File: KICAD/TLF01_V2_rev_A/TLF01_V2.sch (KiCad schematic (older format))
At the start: 52 parts, among them J1 ERK_PWR, J2 Audio_In_Out, J3 EXT_PWR, J4 TP_GND, J5 CUTOFF, Q1 2SC1815, Q10 2SC1815, Q2 2SC1815, Q3 2SC1815, Q4 2SC1815, Q5 2SC1815, Q6 2SC1815, Q7 2SC1815, Q8 2SC1815, Q9 2SC1815, U1 TL072

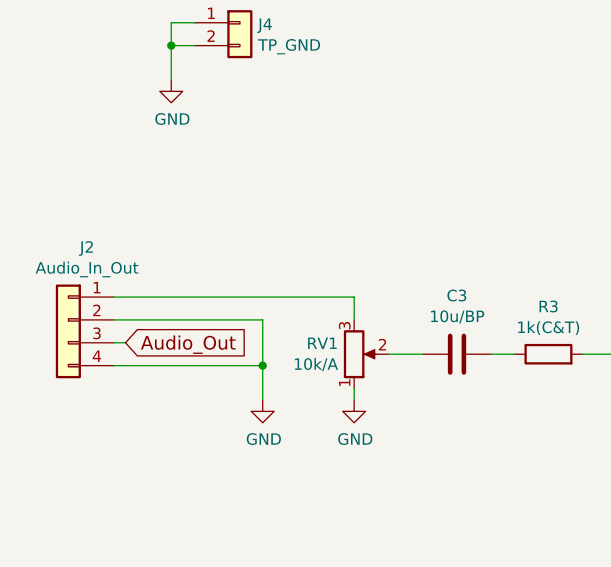
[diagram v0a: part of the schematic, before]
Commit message: Update: PCB Design
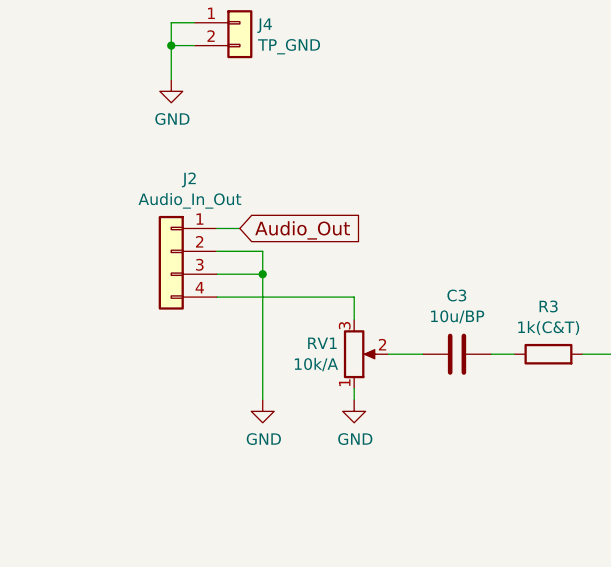
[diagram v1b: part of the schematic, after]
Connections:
- net Audio_Out: now also J2.1 (Pin_1); no longer J2.3 (Pin_3)
- net GND: now also J2.3 (Pin_3); no longer J2.4 (Pin_4)
- net at RV1.3: now also J2.4 (Pin_4); no longer J2.1 (Pin_1)
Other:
- moved on the sheet: J2
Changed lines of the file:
@@
 	1    0    0    -1
 $EndComp
-Wire Wire Line
-	2200 5350 2200 5550
 $Comp
 L power:GND #PWR011
@@
 L Connector_Generic:Conn_01x04 J2
 U 1 1 5F44F858
-P 1350 5350
-F 0 "J2" H 1268 5667 50  0000 C CNN
-F 1 "Audio_In_Out" H 1268 5576 50  0000 C CNN
-F 2 "Connector_JST:JST_XH_B4B-XH-A_1x04_P2.50mm_Vertical" H 1350 5350 50  0001 C CNN
-F 3 "~" H 1350 5350 50  0001 C CNN
-	1    1350 5350
+P 1800 5050
+F 0 "J2" H 1718 5367 50  0000 C CNN
+F 1 "Audio_In_Out" H 1718 5276 50  0000 C CNN
+F 2 "Connector_JST:JST_XH_B4B-XH-A_1x04_P2.50mm_Vertical" H 1800 5050 50  0001 C CNN
+F 3 "~" H 1800 5050 50  0001 C CNN
+	1    1800 5050
 	-1   0    0    -1
 $EndComp
-Text GLabel 1600 5450 2    59   Input ~ 0
+Text GLabel 2100 4950 2    59   Input ~ 0
 Audio_Out
 Wire Wire Line
-	1550 5350 2200 5350
-Wire Wire Line
-	1550 5250 2600 5250
-Wire Wire Line
-	1600 5450 1550 5450
-Wire Wire Line
-	1550 5550 2200 5550
-Connection ~ 2200 5550
-Wire Wire Line
-	2200 5550 2200 5700
+	2000 4950 2100 4950
+Wire Wire Line
+	2000 5050 2200 5050
+Wire Wire Line
+	2200 5050 2200 5150
+Wire Wire Line
+	2600 5250 2000 5250
+Wire Wire Line
+	2000 5150 2200 5150
+Connection ~ 2200 5150
+Wire Wire Line
+	2200 5150 2200 5700
 $EndSCHEMATC
